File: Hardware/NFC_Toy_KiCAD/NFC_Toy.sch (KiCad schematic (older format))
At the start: 48 parts, among them J1 Pad, J2 Pad, J3 JLink_Mini, U1 TPS61032, U19 MIC5225, U2 STM32L0-LQFP48, U3 LIS3DH

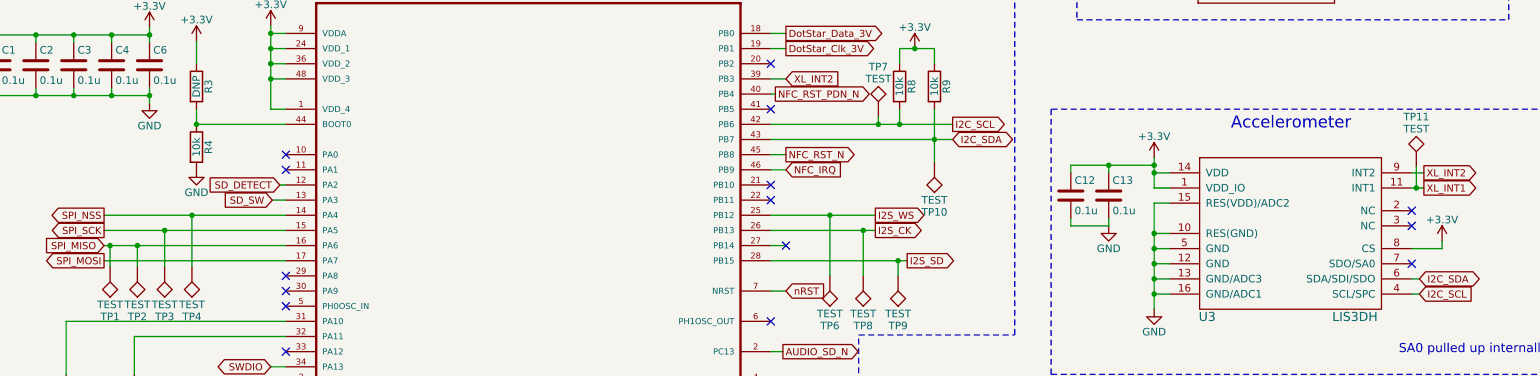
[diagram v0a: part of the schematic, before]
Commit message: First pass layout complete
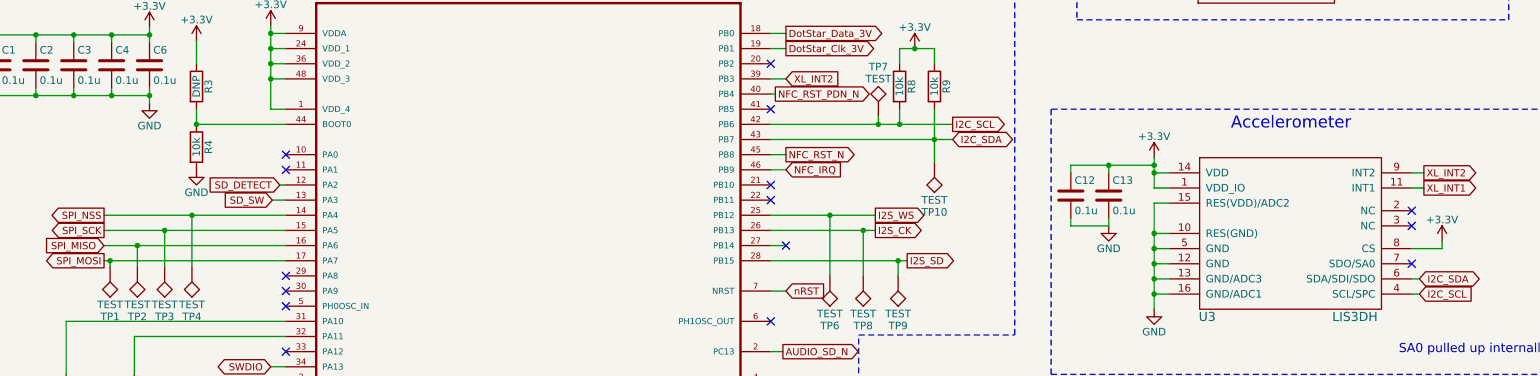
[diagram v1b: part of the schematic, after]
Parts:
- removed TP11: TEST, NFC_Toy_Lib:Test_Point, symbol TEST
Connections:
- net SPI_MISO: no longer TP1.1
- net SPI_MOSI: now also TP1.1
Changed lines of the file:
@@
 	6700 5730 6700 5630
 Connection ~ 6700 5630
-Connection ~ 10120 5150
 Connection ~ 2560 2530
 Wire Notes Line
@@
 	1680 5670 1680 5530
 Connection ~ 1680 5530
-Wire Wire Line
-	1500 5670 1500 5530
-Connection ~ 1500 5530
 $Comp
 L TEST TP5
@@
 	1    0    0    -1
 $EndComp
-$Comp
-L TEST TP11
-U 1 1 5AD3A341
-P 10120 5010
-F 0 "TP11" H 10120 5310 50  0000 C BNN
-F 1 "TEST" H 10120 5260 50  0000 C CNN
-F 2 "NFC_Toy_Lib:Test_Point" H 10120 5010 50  0001 C CNN
-F 3 "" H 10120 5010 50  0001 C CNN
-	1    10120 5010
-	1    0    0    -1
-$EndComp
-Wire Wire Line
-	10120 5010 10120 5150
 NoConn ~ 5860 4330
 NoConn ~ 5860 6030
@@
 Wire Wire Line
 	5960 5030 5860 5030
+Wire Wire Line
+	1500 5670 1500 5630
+Connection ~ 1500 5630
 $EndSCHEMATC

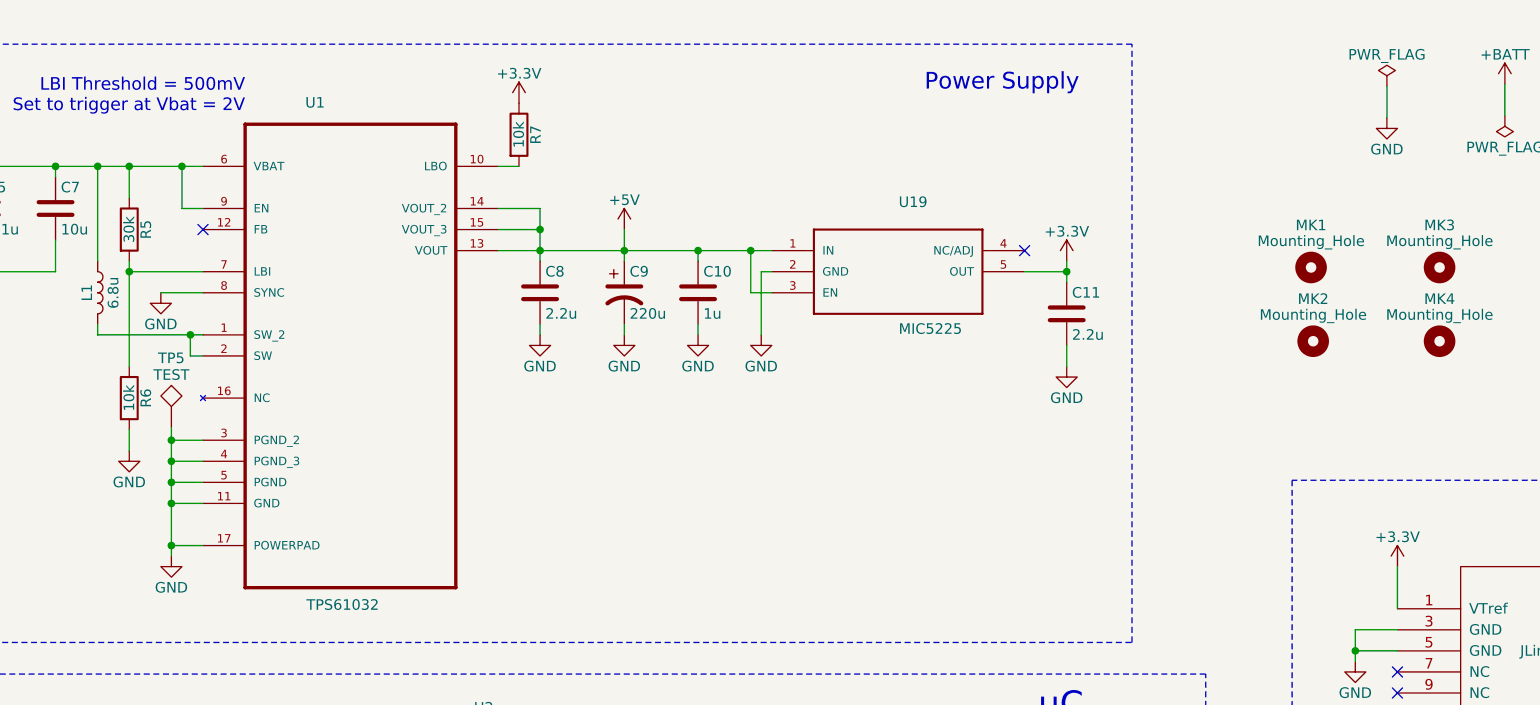
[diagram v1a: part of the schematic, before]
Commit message: Preliminary layout complete
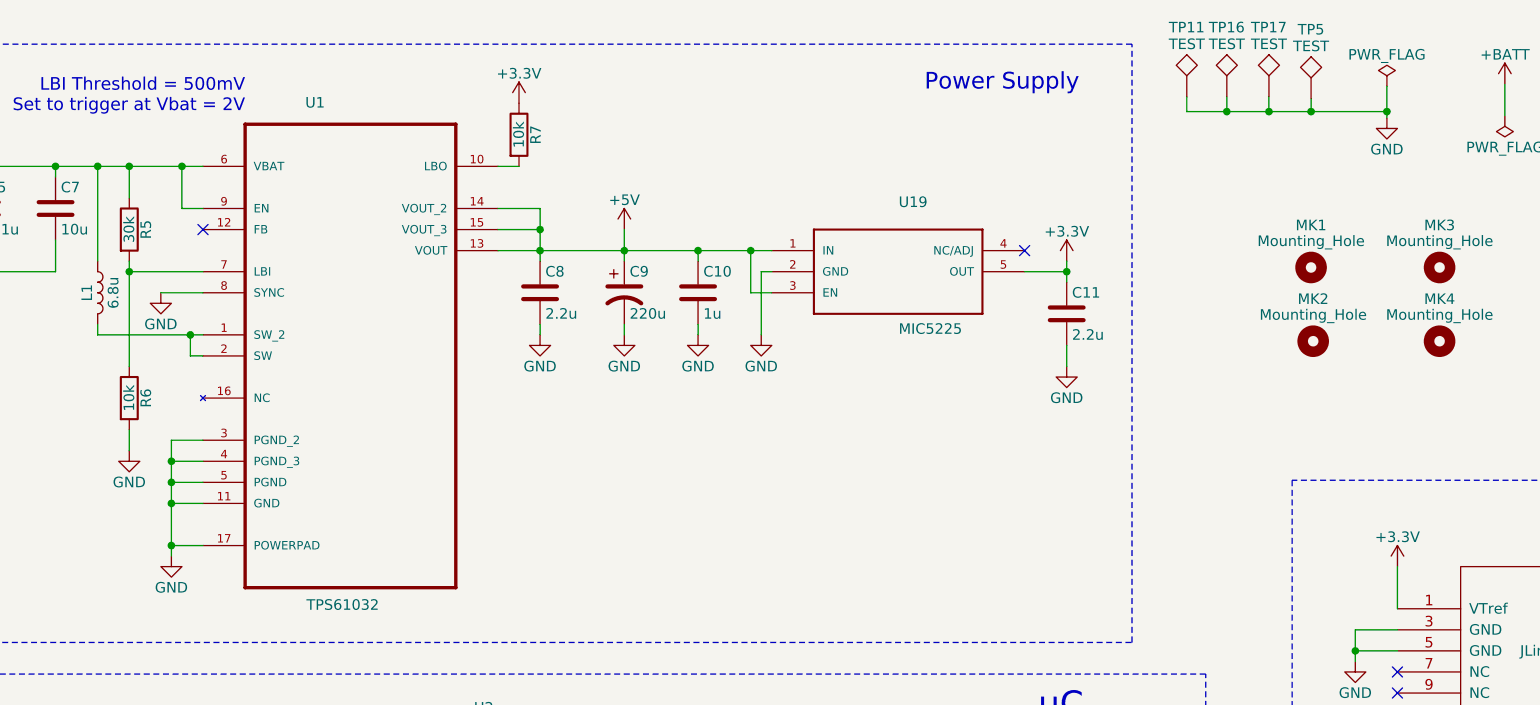
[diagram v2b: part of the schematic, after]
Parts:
- added TP11, TP16, TP17: TEST, NFC_Toy_Lib:Test_Point, symbol TEST
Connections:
- net GND: now also TP11.1, TP16.1, TP17.1
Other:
- moved on the sheet: TP5
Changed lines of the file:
@@
 	2510 1830 2710 1830
-Wire Wire Line
-	2710 2530 2560 2530
-Wire Wire Line
-	2560 2470 2560 3080
-Wire Wire Line
-	2710 2630 2560 2630
-Connection ~ 2560 2630
 Wire Wire Line
 	2710 2730 2560 2730
 Connection ~ 2560 2730
 Wire Wire Line
-	2710 2830 2560 2830
+	2560 2830 2710 2830
 Connection ~ 2560 2830
 Wire Wire Line
-	2710 3030 2560 3030
+	2560 3030 2710 3030
 Connection ~ 2560 3030
 Connection ~ 1460 1230
@@
 	6700 5730 6700 5630
 Connection ~ 6700 5630
-Connection ~ 2560 2530
 Wire Notes Line
 	660  3640 660  7640
@@
 L TEST TP5
 U 1 1 5AD39F6E
-P 2560 2470
-F 0 "TP5" H 2560 2770 50  0000 C BNN
-F 1 "TEST" H 2560 2720 50  0000 C CNN
-F 2 "NFC_Toy_Lib:Test_Point" H 2560 2470 50  0001 C CNN
-F 3 "" H 2560 2470 50  0001 C CNN
-	1    2560 2470
+P 7970 910
+F 0 "TP5" H 7970 1210 50  0000 C BNN
+F 1 "TEST" H 7970 1160 50  0000 C CNN
+F 2 "NFC_Toy_Lib:Test_Point" H 7970 910 50  0001 C CNN
+F 3 "" H 7970 910 50  0001 C CNN
+	1    7970 910
 	1    0    0    -1
 $EndComp
@@
 	1500 5670 1500 5630
 Connection ~ 1500 5630
+Wire Wire Line
+	2560 2530 2560 3080
+$Comp
+L TEST TP17
+U 1 1 5AE3537D
+P 7770 900
+F 0 "TP17" H 7770 1200 50  0000 C BNN
+F 1 "TEST" H 7770 1150 50  0000 C CNN
+F 2 "NFC_Toy_Lib:Test_Point" H 7770 900 50  0001 C CNN
+F 3 "" H 7770 900 50  0001 C CNN
+	1    7770 900
+	1    0    0    -1
+$EndComp
+$Comp
+L TEST TP16
+U 1 1 5AE3544B
+P 7570 900
+F 0 "TP16" H 7570 1200 50  0000 C BNN
+F 1 "TEST" H 7570 1150 50  0000 C CNN
+F 2 "NFC_Toy_Lib:Test_Point" H 7570 900 50  0001 C CNN
+F 3 "" H 7570 900 50  0001 C CNN
+	1    7570 900
+	1    0    0    -1
+$EndComp
+$Comp
+L TEST TP11
+U 1 1 5AE35510
+P 7380 900
+F 0 "TP11" H 7380 1200 50  0000 C BNN
+F 1 "TEST" H 7380 1150 50  0000 C CNN
+F 2 "NFC_Toy_Lib:Test_Point" H 7380 900 50  0001 C CNN
+F 3 "" H 7380 900 50  0001 C CNN
+	1    7380 900
+	1    0    0    -1
+$EndComp
+Wire Wire Line
+	7380 900  7380 970
+Wire Wire Line
+	7380 970  8330 970
+Connection ~ 8330 970
+Wire Wire Line
+	7970 910  7970 970
+Connection ~ 7970 970
+Wire Wire Line
+	7770 900  7770 970
+Connection ~ 7770 970
+Wire Wire Line
+	7570 900  7570 970
+Connection ~ 7570 970
+Wire Wire Line
+	2710 2530 2560 2530
+Wire Wire Line
+	2710 2630 2560 2630
+Connection ~ 2560 2630
 $EndSCHEMATC
